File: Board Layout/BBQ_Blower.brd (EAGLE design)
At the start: 84.9 x 75.9 mm, 27 parts, among them IC1 MAX31855RASA+, IC2 MAX31855RASA+, IC3 MAX31855RASA+, J1 PCC-SMP-K-100-R-ROHS, J3 PCC-SMP-K-100-R-ROHS, J4 PCC-SMP-K-100-R-ROHS, Q1 BUZ10, Q2 BUZ10, U1 113990105

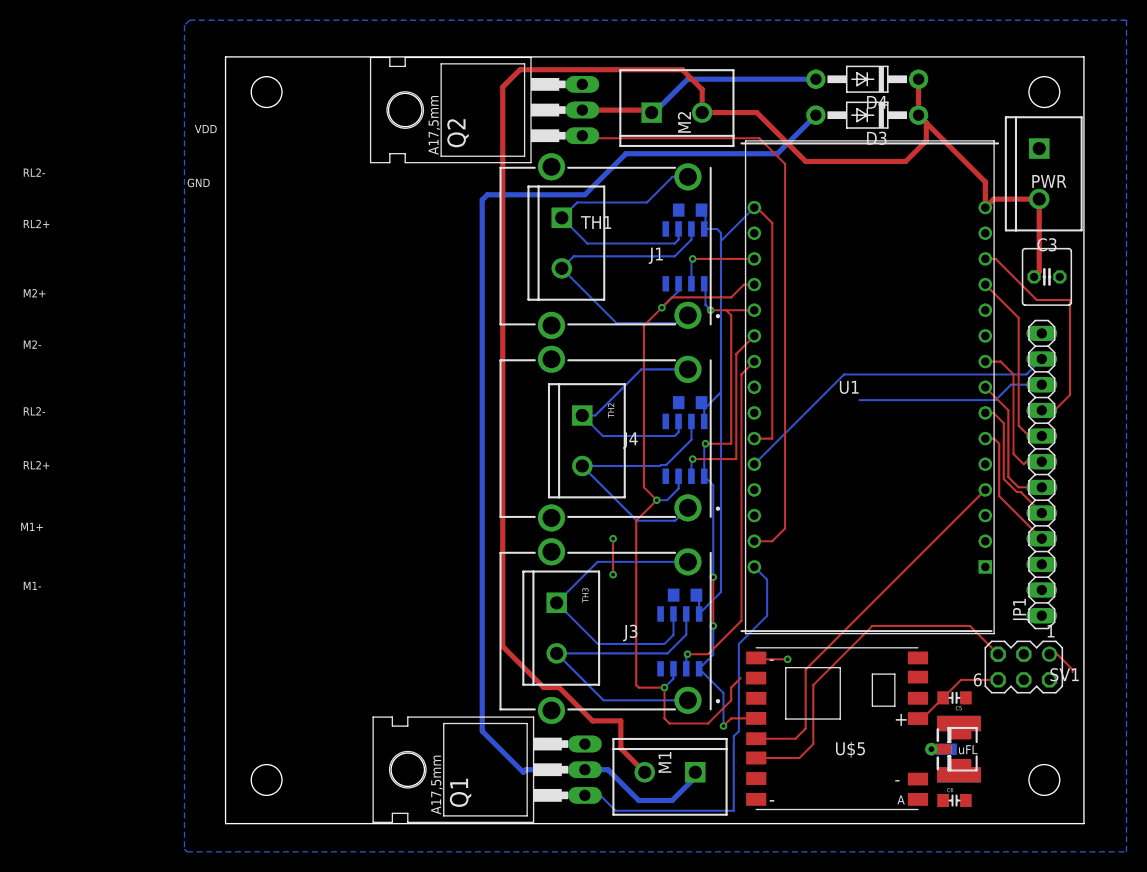
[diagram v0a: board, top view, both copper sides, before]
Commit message: re-arraging
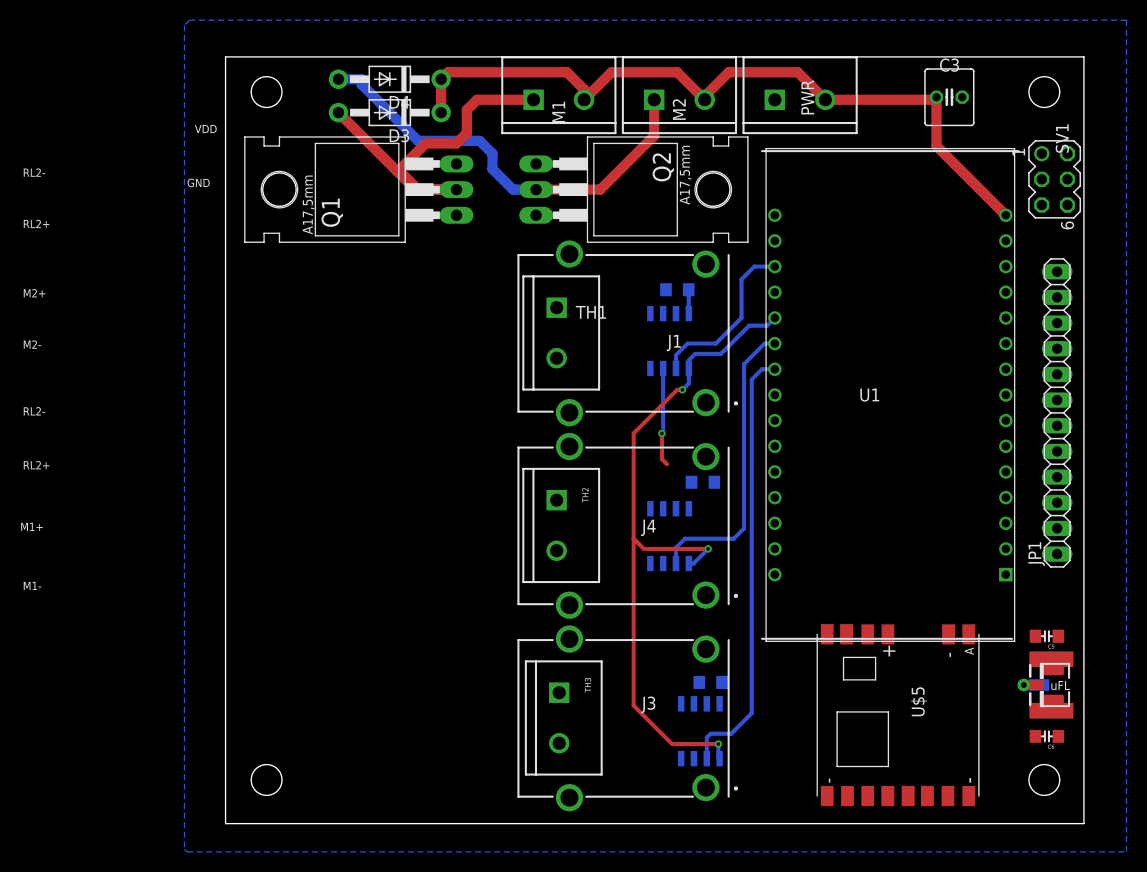
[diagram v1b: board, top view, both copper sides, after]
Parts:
- moved M1 68.4 mm to (35.8, 75.7), turned to 0 degrees
- moved Q1 58.8 mm to (21.8, 66.8)
- moved SV1 48.4 mm to (87.4, 67.8), turned to 270 degrees
- moved D3 47.2 mm to (21.6, 74.4)
- moved D4 47.2 mm to (21.6, 77.7)
- moved PWR 26.6 mm to (59.7, 75.7), turned to 0 degrees
- moved C3 20.2 mm to (77.0, 75.9)
- moved Q2 11.3 mm to (42.4, 66.8), turned to 270 degrees
- moved J$2 11.1 mm to (89.4, 17.8)
- moved C6 11.1 mm to (86.6, 12.7), turned to 180 degrees
- moved C5 11.0 mm to (86.6, 22.6)
- moved IC1 9.12 mm to (52.3, 13.2)
- moved C2 9.00 mm to (53.3, 18.0)
- moved TH1 8.90 mm to (38.1, 55.1)
- moved TH3 8.89 mm to (38.4, 17.0)
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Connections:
- removed net RELAY_1: U1.28
- removed net RELAY_2: U1.27
- new net DIO5: U$5.DIO5, U1.5
- new net N$1: U1.3
- net D2: no longer U1.5
- net D4: no longer U1.26
- net DIO0: now also U1.28
- net DIO1: now also U1.27
- net DIO2: now also U1.26
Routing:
- net 3V3: track 107.6 -> 2.37 mm
- net VDD: track 155.5 -> 73.7 mm
- net BLOWER2: track 114.7 -> 38.6 mm
- net SO: track 75.0 -> 9.74 mm, vias 3 -> 1
- net BLOWER_2: track 60.9 -> 0.00 mm
- net RST: track 56.8 -> 0.00 mm
- net BLOWER_1: track 41.4 -> 0.00 mm
- net CS_LORA: track 36.3 -> 0.00 mm
- net D4: track 32.8 -> 0.00 mm
- net T1+: track 30.6 -> 0.00 mm
- net T1-: track 30.4 -> 0.00 mm
- net T3+: track 30.1 -> 0.00 mm
- net T3-: track 28.0 -> 0.00 mm
- net T2+: track 26.9 -> 0.00 mm
- net T2-: track 23.9 -> 0.00 mm
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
